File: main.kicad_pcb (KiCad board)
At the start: 2 copper layers, 120 x 100 mm, 21 parts, among them J1 Conn_01x01_Female, J2 Conn_01x01_Female, J3 Conn_01x01_Female, J4 Conn_01x01_Female, J5 Conn_01x01_Female, J6 Conn_01x01_Female, J7 Conn_Coaxial, Q1 AOT2618

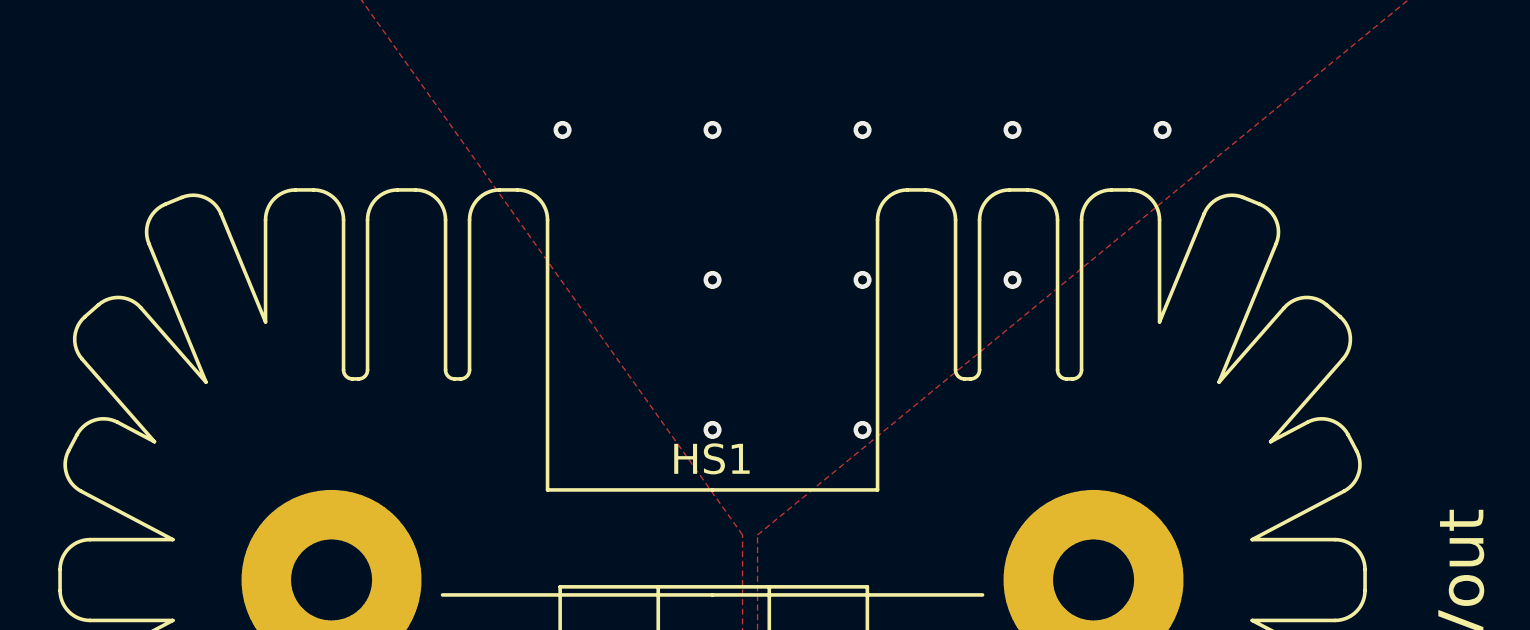
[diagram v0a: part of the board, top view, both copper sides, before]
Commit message: Updated libs (#2)
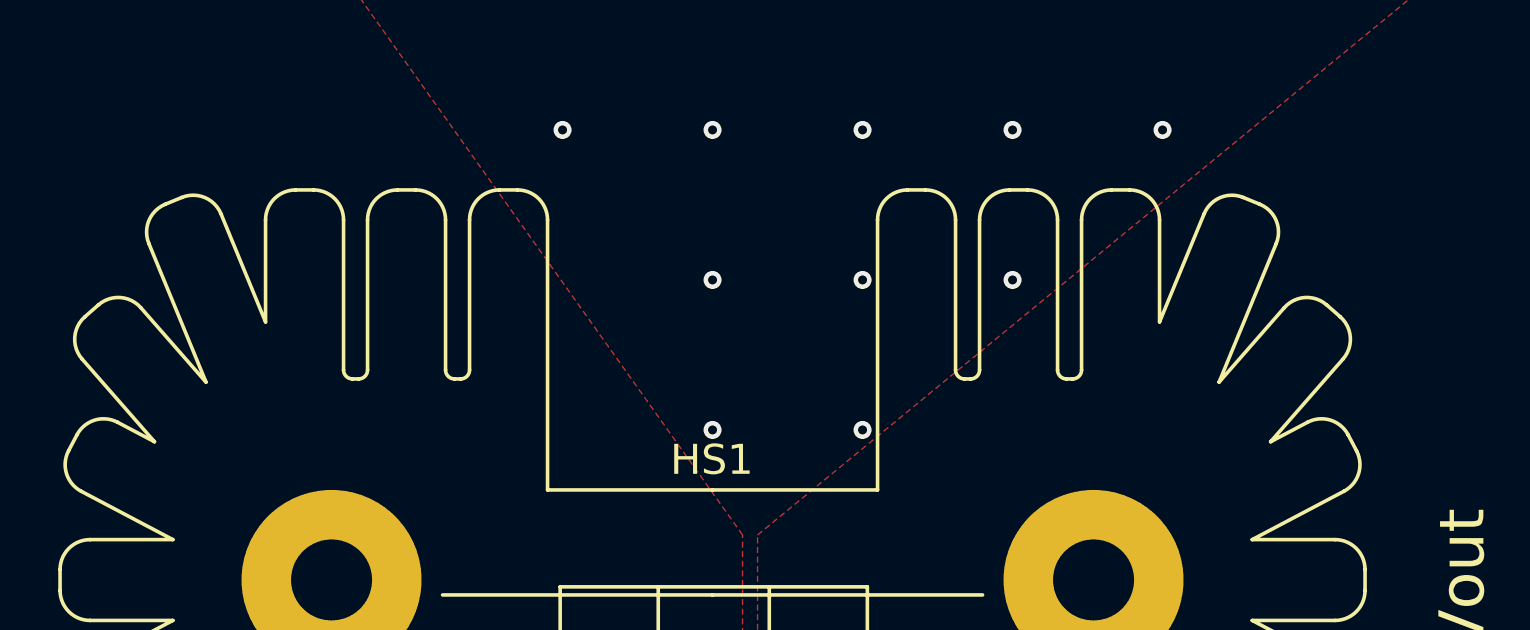
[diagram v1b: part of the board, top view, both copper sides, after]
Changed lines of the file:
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@@
 	(net 7 "unconnected-(HS1-Pad1)")
 	(net 8 "Net-(J3-Pin_1)")
+	(net 9 "unconnected-(HS1-Pad1)_1")
 	(footprint "Capacitor_THT:CP_Radial_D10.0mm_P5.00mm"
 		(layer "F.Cu")
@@
 			)
 		)
-		(property "Description" ""
+		(property "Description" "Generic connector, single row, 01x01, script generated"
 			(at 0 0 0)
 			(unlocked yes)
@@
 			)
 		)
-		(property ki_fp_filters "Connector*:*")
+		(property ki_fp_filters "Connector*:*_1x??_*")
 		(sheetname "Root")
 		(sheetfile "main.kicad_sch")
@@
 			)
 		)
-		(property "Description" ""
+		(property "Description" "Generic connector, single row, 01x01, script generated"
 			(at 0 0 0)
 			(unlocked yes)
@@
 			)
 		)
-		(property ki_fp_filters "Connector*:*")
+		(property ki_fp_filters "Connector*:*_1x??_*")
 		(sheetname "Root")
 		(sheetfile "main.kicad_sch")
@@
 			)
 		)
-		(property "Description" ""
+		(property "Description" "Open Hardware logo, small"
 			(at 0 0 0)
 			(layer "F.Fab")
@@
 			)
 		)
-		(property "exclude_from_bom" ""
-			(at 0 0 0)
-			(layer "F.Fab")
-			(hide yes)
-			(effects
-				(font
-					(size 1 1)
-					(thickness 0.15)
-				)
-			)
-		)
 		(sheetname "Root")
 		(sheetfile "main.kicad_sch")
@@
 			)
 		)
-		(property "Description" ""
+		(property "Description" "Generic connector, single row, 01x01, script generated"
 			(at 0 0 0)
 			(unlocked yes)
@@
 			)
 		)
-		(property ki_fp_filters "Connector*:*")
+		(property ki_fp_filters "Connector*:*_1x??_*")
 		(sheetname "Root")
 		(sheetfile "main.kicad_sch")
@@
 			)
 		)
-		(property "Datasheet" " ~"
+		(property "Datasheet" ""
 			(at 0 0 90)
 			(layer "F.Fab")
@@
 			)
 		)
-		(property "Description" ""
+		(property "Description" "coaxial connector (BNC, SMA, SMB, SMC, Cinch/RCA, LEMO, ...)"
 			(at 0 0 90)
 			(layer "F.Fab")
@@
 			)
 		)
-		(property ki_fp_filters "*BNC* *SMA* *SMB* *SMC* *Cinch* *LEMO*")
+		(property ki_fp_filters "*BNC* *SMA* *SMB* *SMC* *Cinch* *LEMO* *UMRF* *MCX* *U.FL*")
 		(sheetname "Root")
 		(sheetfile "main.kicad_sch")
@@
 			)
 		)
+		(model "${KIPRJMOD}/footprints_project_specific.3dshapes/bnc_90_1-1337543-0.wrl"
+			(offset
+				(xyz 0 12.54 0)
+			)
+			(scale
+				(xyz 1 1 1)
+			)
+			(rotate
+				(xyz 0 0 180)
+			)
+		)
 	)
 	(footprint "Connector:Banana_Cliff_FCR7350B_S16N-PC_Horizontal"
@@
 			)
 		)
-		(property "Description" ""
+		(property "Description" "Generic connector, single row, 01x01, script generated"
 			(at 0 0 180)
 			(unlocked yes)
@@
 			)
 		)
-		(property ki_fp_filters "Connector*:*")
+		(property ki_fp_filters "Connector*:*_1x??_*")
 		(sheetname "Root")
 		(sheetfile "main.kicad_sch")
@@
 			)
 		)
-		(property "Description" ""
+		(property "Description" "Generic connector, single row, 01x01, script generated"
 			(at 0 0 180)
 			(unlocked yes)
@@
 			)
 		)
-		(property ki_fp_filters "Connector*:*")
+		(property ki_fp_filters "Connector*:*_1x??_*")
 		(sheetname "Root")
 		(sheetfile "main.kicad_sch")
@@
 		(fp_arc
 			(start -17.691791 -12.749206)
-			(mid -16.926425 -12.74787)
+			(mid -16.926426 -12.74787)
 			(end -16.386175 -12.20573)
 			(stroke
@@
 		(fp_arc
 			(start 18.007467 12.859044)
-			(mid 17.24283 12.892429)
+			(mid 17.242829 12.892428)
 			(end 16.678541 12.375356)
 			(stroke
@@
 		(fp_arc
 			(start 19.058317 -9.075185)
-			(mid 19.74445 -9.414276)
+			(mid 19.74445 -9.414242)
 			(end 20.469421 -9.168911)
 			(stroke
@@
 		(fp_arc
 			(start 19.834479 -5.256572)
-			(mid 20.59659 -5.327292)
+			(mid 20.596584 -5.327302)
 			(end 21.185447 -4.838378)
 			(stroke
@@
 		(fp_arc
 			(start 9.39953 -11.8)
-			(mid 9.604557 -12.294964)
+			(mid 9.604561 -12.294969)
 			(end 10.09953 -12.5)
 			(stroke
@@
 		(fp_arc
 			(start 12.79953 -11.8)
-			(mid 13.004557 -12.294964)
+			(mid 13.004551 -12.294999)
 			(end 13.49953 -12.5)
 			(stroke
@@
 		(fp_arc
 			(start 13.725181 -12.49953)
-			(mid 14.203473 -12.285811)
+			(mid 14.203509 -12.285818)
 			(end 14.39953 -11.8)
 			(stroke
@@
 		(fp_arc
 			(start 14.30047 11.8)
-			(mid 14.095443 12.294964)
+			(mid 14.095449 12.294999)
 			(end 13.60047 12.5)
 			(stroke
@@
 			(layers "*.Cu" "*.Mask")
 			(remove_unused_layers no)
-			(net 7 "unconnected-(HS1-Pad1)")
+			(net 9 "unconnected-(HS1-Pad1)_1")
 			(pintype "passive+no_connect")
 		)
@@
 			)
 		)
-		(property "Description" ""
+		(property "Description" "Generic connector, single row, 01x01, script generated"
 			(at 0 0 0)
 			(unlocked yes)
@@
 			)
 		)
-		(property ki_fp_filters "Connector*:*")
+		(property ki_fp_filters "Connector*:*_1x??_*")
 		(sheetname "Root")
 		(sheetfile "main.kicad_sch")
